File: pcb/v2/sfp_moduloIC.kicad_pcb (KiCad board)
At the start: 4 copper layers, 60 x 84.5 mm, 149 parts, among them J1 SPI, J2 FTDI, J3 SWD, J4 RATE, J5 DIS, J6 SFP, J7 POWER, J8 IN, Q1 BC848, Q2 BC848, Q3 BC848, SW1 RESET, U1 MCP6002-xSN, U2 W5500, U3 STM32F103C8Tx, U4 RTL8213B-CG, U5 Ai-Thinker-Ra-01, Y1 25mhz, Y2 25mhz

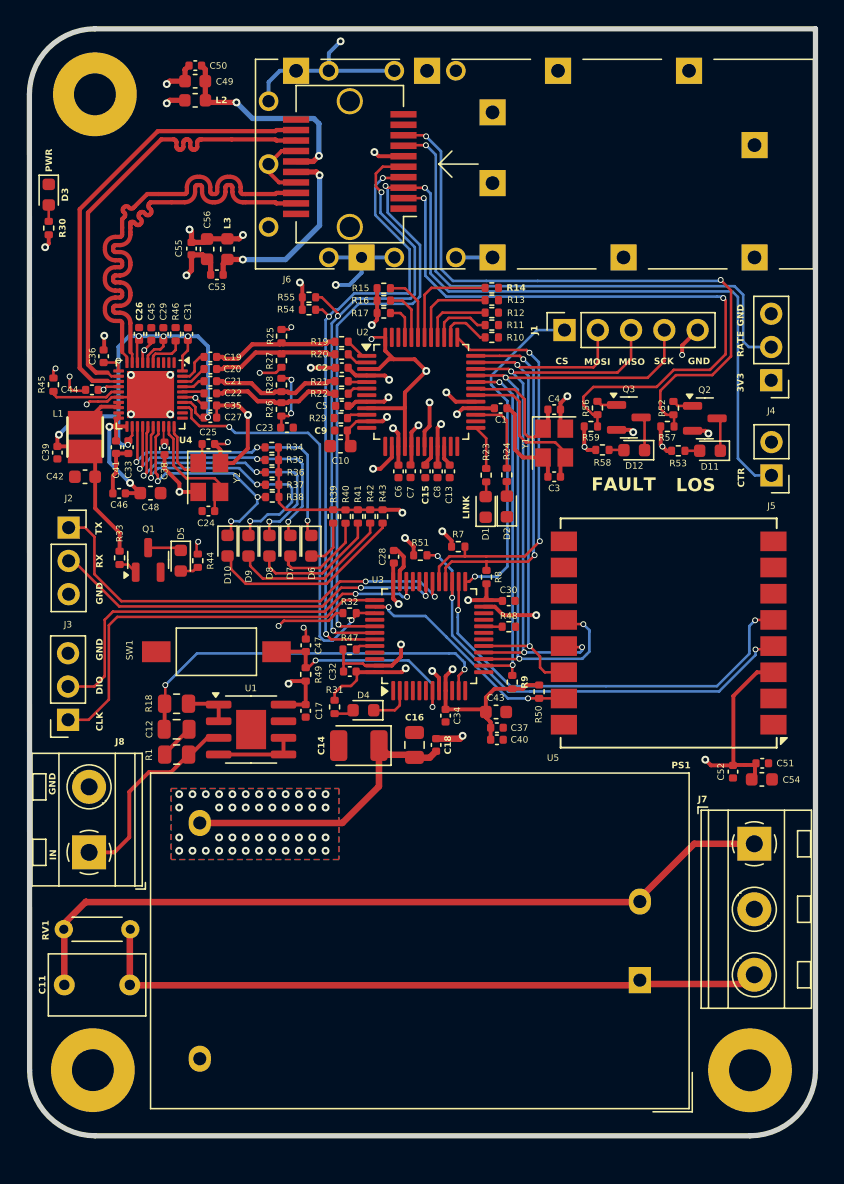
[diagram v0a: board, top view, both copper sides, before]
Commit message: v4.1
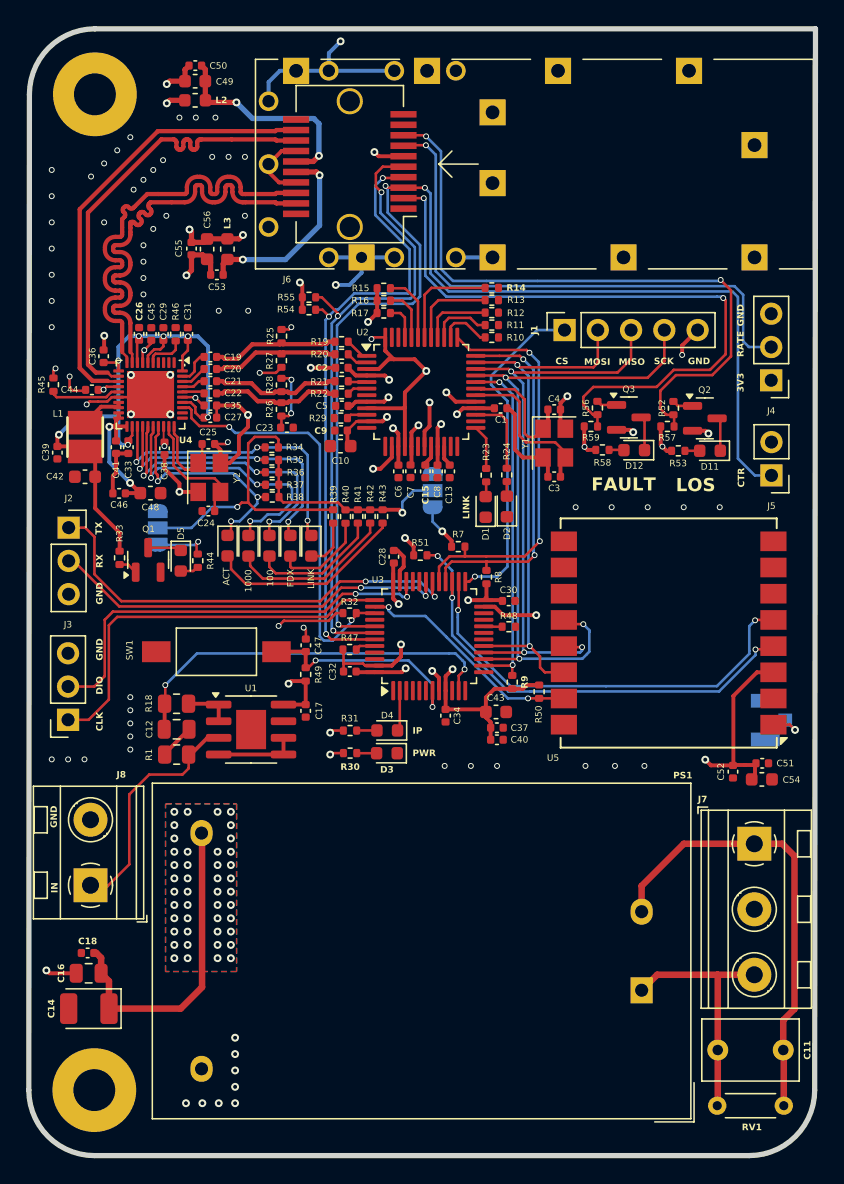
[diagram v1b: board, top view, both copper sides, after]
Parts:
- removed the H2 at (170.4, 130.5)
- added J11: ANT, KiCad3:CONUFL001SMDT, B.Cu at (171.5, 103.7)
- added JP1: SEL, Jumper:SolderJumper-3_P1.3mm_Open_RoundedPad1.0x1.5mm, B.Cu at (125.1, 89.0)
- added JP2: SEL, Jumper:SolderJumper-3_P1.3mm_Open_RoundedPad1.0x1.5mm, B.Cu at (146.1, 86.2)
- moved D3 49.9 mm to (142.6, 106.2), turned to 180 degrees
- moved RV1 46.8 mm to (167.9, 133.2), turned to 0 degrees
- moved R30 46.2 mm to (139.8, 106.2), turned to 180 degrees
- moved C11 45.2 mm to (167.9, 128.9), turned to 0 degrees
- moved C18 31.0 mm to (119.8, 121.5), turned to 180 degrees
- moved C16 30.4 mm to (119.9, 123.0), turned to 180 degrees
- moved C14 28.8 mm to (119.9, 125.7)
- moved J8 2.51 mm to (120.0, 116.3)
- moved D4 2.38 mm to (142.7, 104.5)
- moved R31 2.15 mm to (139.8, 104.5), turned to 180 degrees
- moved H2 1.53 mm to (120.3, 132.0)
- moved PS1 0.78 mm to (162.1, 124.3)
- renumbered H3 to H2
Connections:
- R34 pad 1: +3V3 -> /DISAUTO
- R35 pad 1: +3V3 -> /CONFIG
- R36 pad 1: +3V3 -> /CONFIG
- R37 pad 1: +3V3 -> /CONFIG
- R38 pad 1: +3V3 -> /CONFIG
- R39 pad 1: +3V3 -> /DISAUTO
- R40 pad 1: +3V3 -> /CONFIG
- R41 pad 1: +3V3 -> /CONFIG
- R42 pad 1: +3V3 -> /CONFIG
- R43 pad 1: +3V3 -> /CONFIG
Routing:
- net /L: track 52.5 -> 21.1 mm
- net /N: track 59.1 -> 34.9 mm
- net /DISAUTO: track 0.00 -> 22.1 mm, vias 0 -> 1
- net /CONFIG: track 0.00 -> 16.3 mm, vias 0 -> 1
- net +3V3: track 158.6 -> 149.1 mm
- net /ANT: track 0.00 -> 2.88 mm, vias 0 -> 1
- net /IN: track 15.4 -> 18.2 mm
- net GND: track 141.1 -> 141.2 mm, vias 30 -> 88
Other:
- board size 60 x 84.5 mm -> 60.1 x 86 mm
- board text added: "100"
- board text added: "1000"
- board text added: "ACT"
- board text added: "DIS"
- board text added: "FDX"
- board text added: "IP"
- board text added: "SEL"
